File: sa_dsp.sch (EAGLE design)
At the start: 327 parts, among them CN1 uSD, CN3 2X5_HEADER, Q3 2N7002, Q4 2N7002, SW1 1825910-7, U1 PGA2311, U10 LME49720, U11 PGA2311, U12 LME49720, U13 LME49720, U14 PCM1754, U15 LME49720, U16 PGA2311, U17 LME49720, U18 LME49720, U19 PCM1754, U2 LM317, U20 LME49720, U21 7 SEG, U22 74HC164A, U23 PCM2707PJT, U24 PCM2707PJT, U25 7 SEG, U26 74HC164A, U27 LM337, U28 LM317, U29 7 SEG, U3 OSD3358-512M-BSM, U30 74HC164A, U31 100MHz, U4 LME49720, U5 LME49720, U6 10CL016YF484C6G, U7 7 SEG, U8 74HC164A, U9 PCM1754

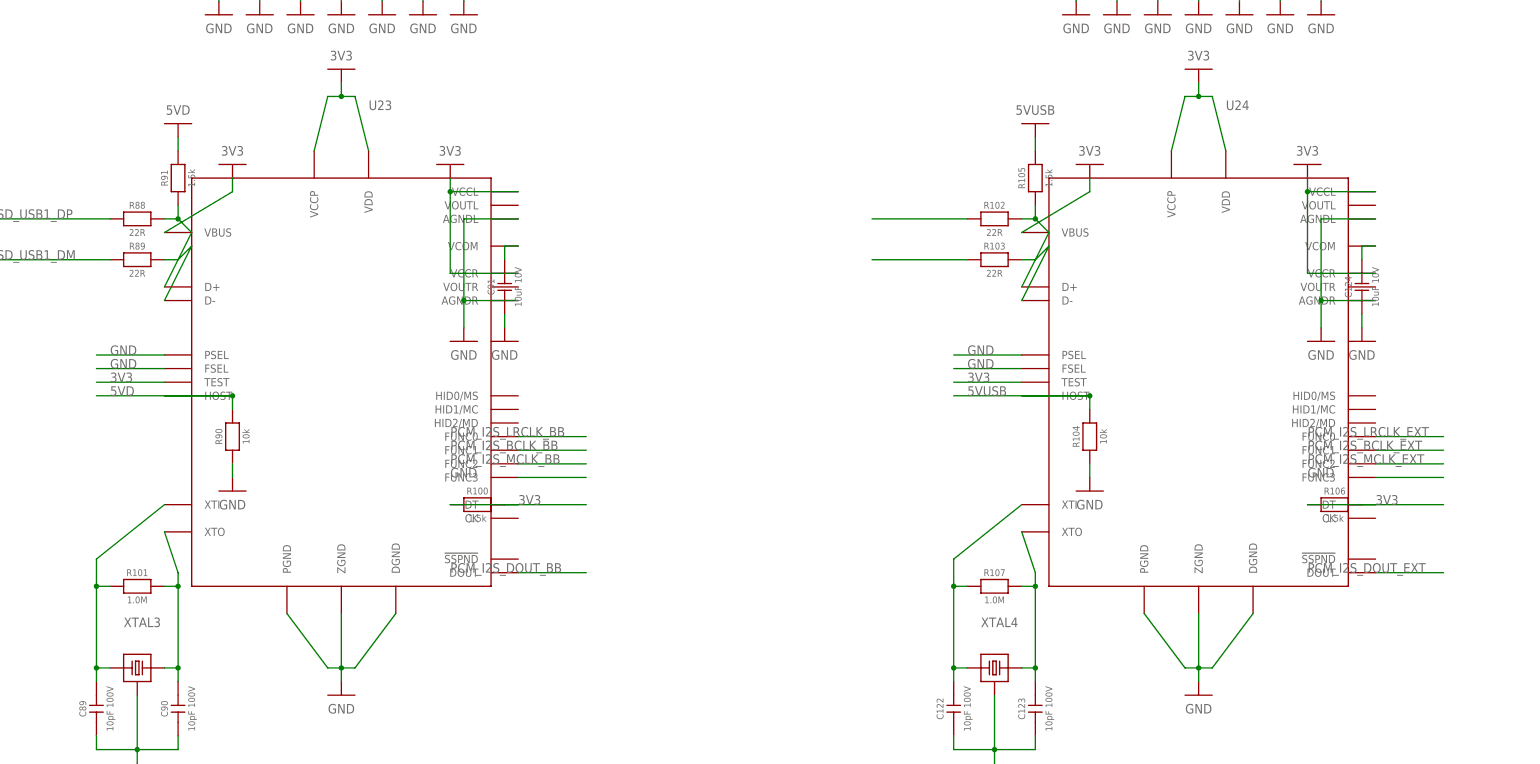
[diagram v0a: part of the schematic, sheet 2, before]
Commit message: Libraies sorted
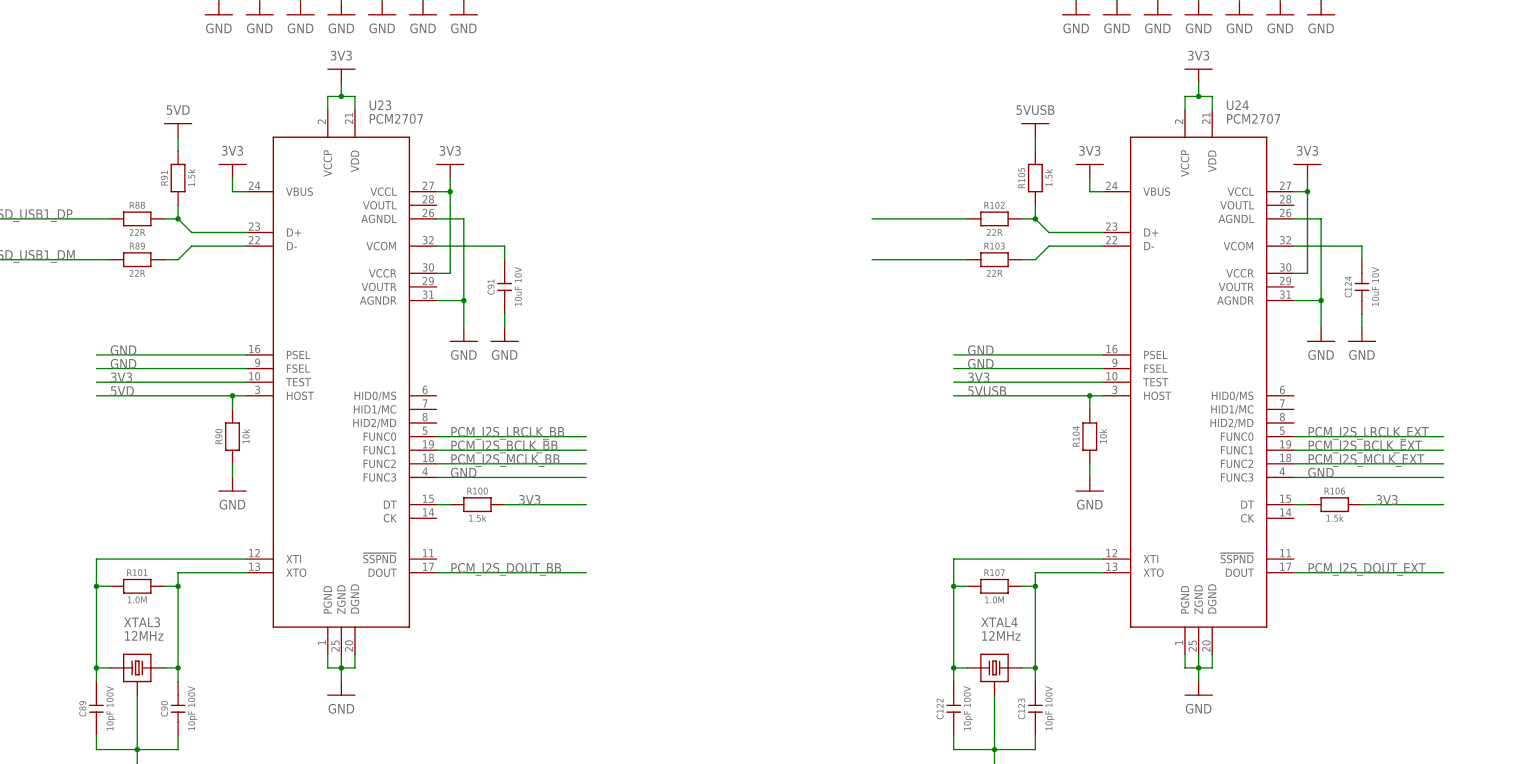
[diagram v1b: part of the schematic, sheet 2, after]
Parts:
- CN3: value 2X5_HEADER -> 2X5 HEADER
- U23, U24: value PCM2707PJT -> PCM2707
- XTAL3, XTAL4: value ABM8-12.000MHZ-B2-T -> 12MHz
